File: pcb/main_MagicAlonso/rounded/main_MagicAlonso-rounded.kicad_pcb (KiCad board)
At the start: 2 copper layers, 89 x 113.2 mm, 103 parts, among them J1 XT30PW-M, J10 ESC1, J11 ESC2, J12 ESC3, J13 USB_C_Receptacle_USB2.0_16P, J14 UART_Out, J15 ESC_VM, J16 USB_B_Micro, J2 MPU6050, J4 Encoder1, J5 Encoder2, J9 Sensors, Q1 IRLML2502, SW1 Power_SW, SW2 EN_Push, SW3 Boot_SW, SW4 BUTTON_Push, U1 ESP32-WROOM-32E, U2 ACS712-30A, U3 ACS712-20A, U4 CH340C, U6 Mini360

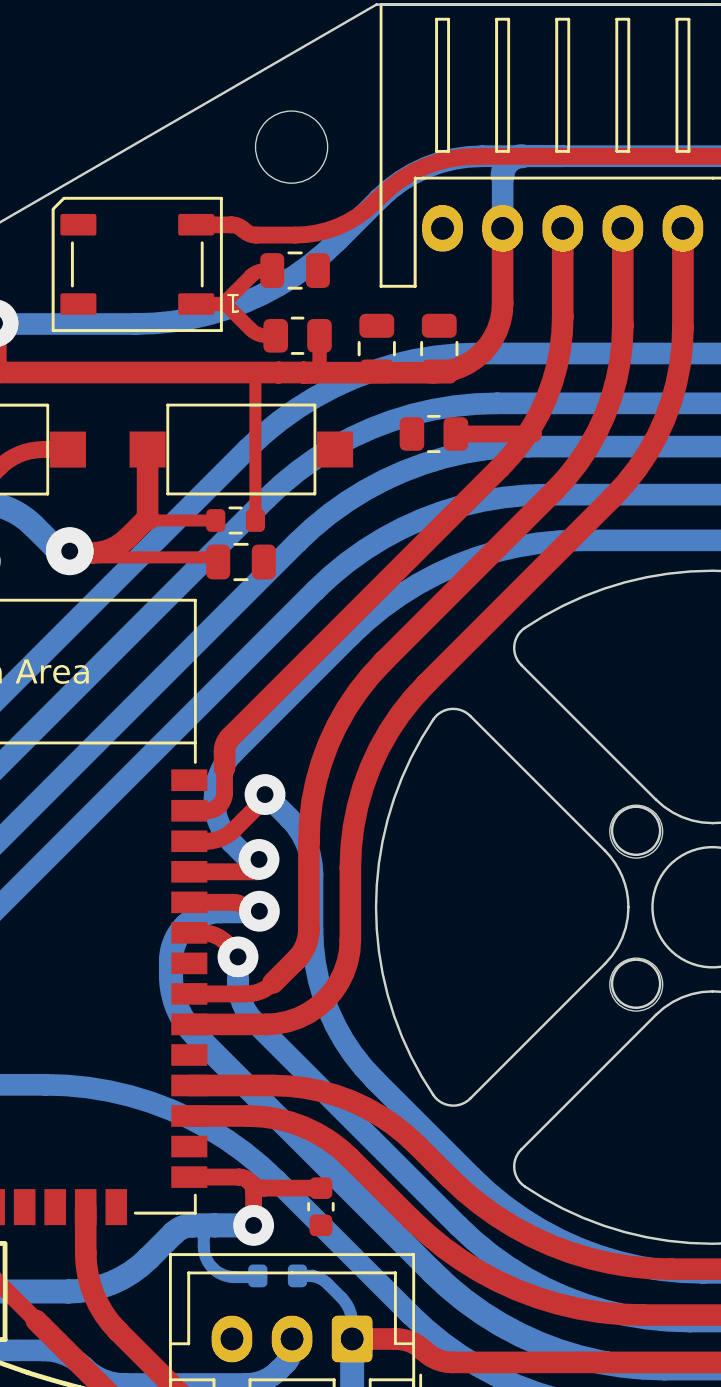
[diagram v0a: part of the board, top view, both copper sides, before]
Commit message: sensors pcb update
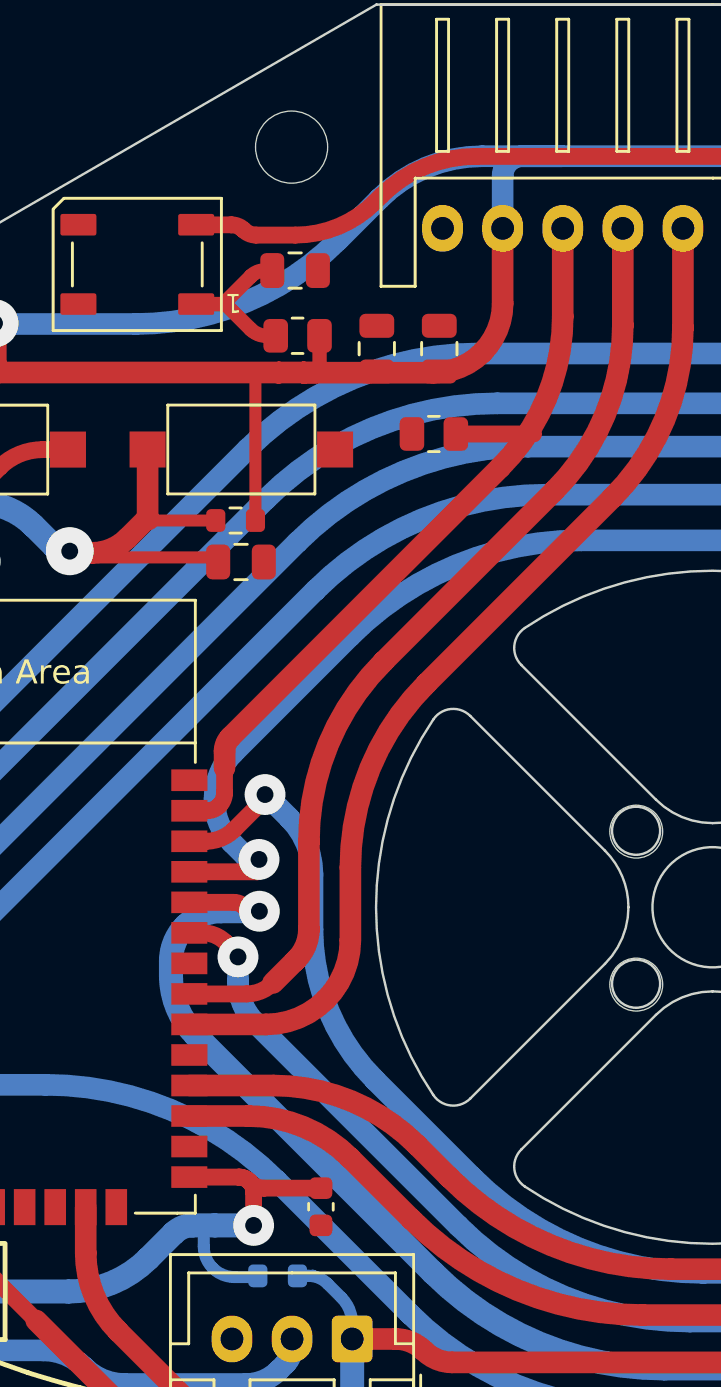
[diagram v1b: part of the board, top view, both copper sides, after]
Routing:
- net /BOOT: track 25.2 -> 24.5 mm
